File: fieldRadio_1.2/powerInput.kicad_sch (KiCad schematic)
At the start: 7 parts, among them Q21 IRF9540, U10 LM1086-5.0

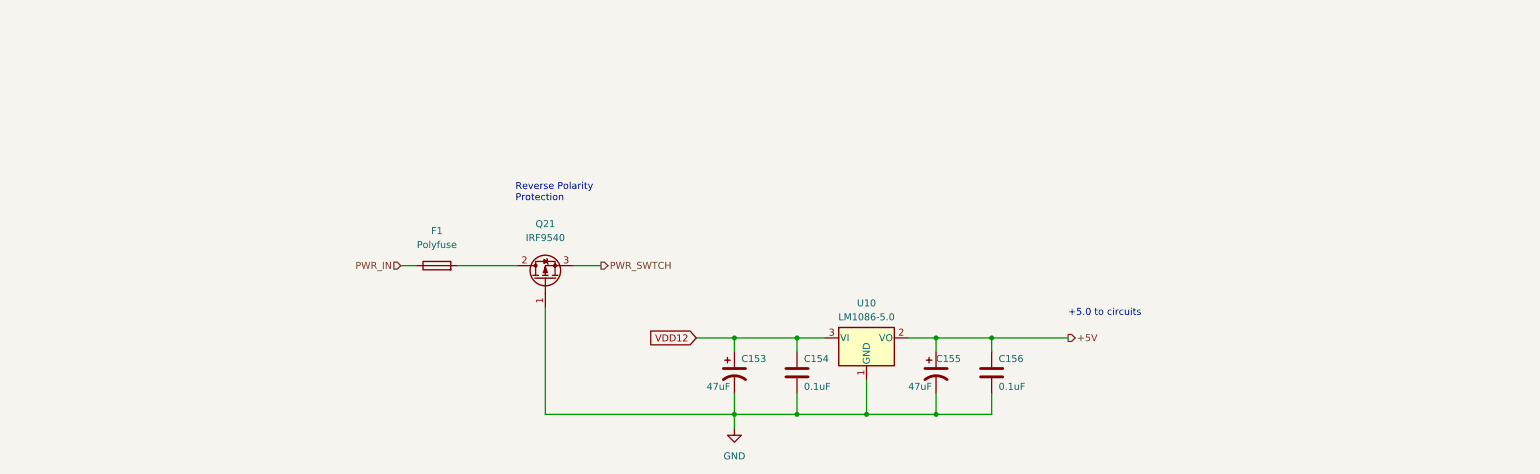
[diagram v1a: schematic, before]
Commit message: Working on fieldRadio_1.2 schematics
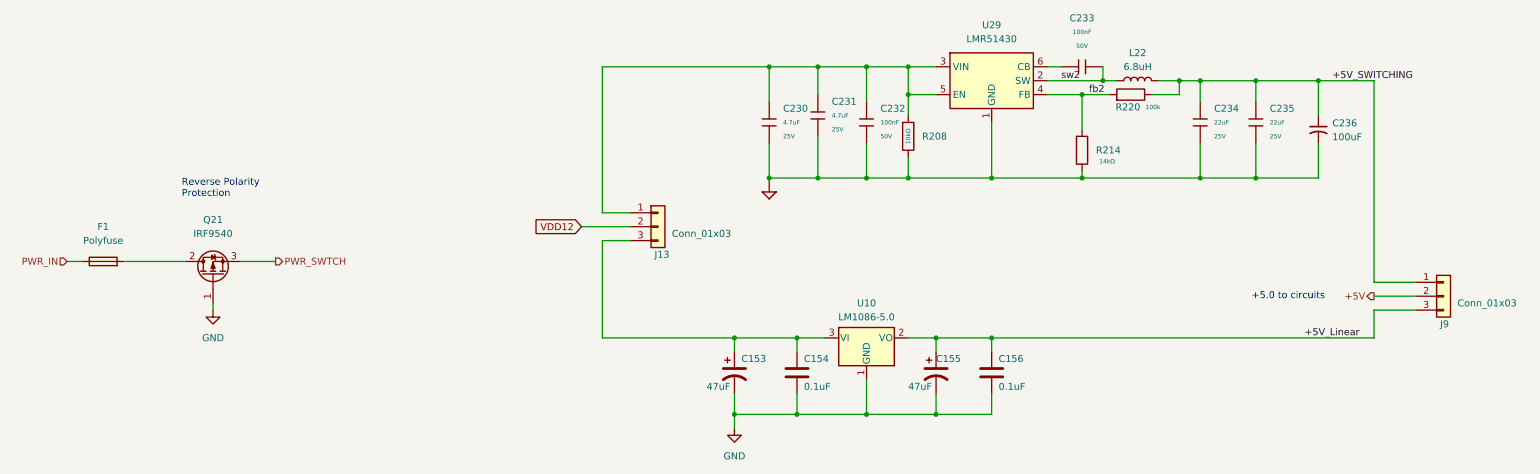
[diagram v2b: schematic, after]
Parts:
- added C230, C231: 4.7uF, PCM_JLCPCB:C_0805, symbol PCM_JLCPCB-Capacitors:0805,4.7uF
- added C232, C233: 100nF, PCM_JLCPCB:C_0603, symbol PCM_JLCPCB-Capacitors:0603,100nF
- added C234, C235: 22uF, PCM_JLCPCB:C_0805, symbol PCM_JLCPCB-Capacitors:0805,22uF
- added C236: 100uF, Capacitor_SMD:C_Elec_6.3x5.8, symbol Device:C_Small_US
- added J13, J9: Conn_01x03, Connector_Wire:SolderWire-0.75sqmm_1x03_P4.8mm_D1.25mm_OD2.3mm, symbol Connector_Generic:Conn_01x03
- added L22: 6.8uH, Inductor_SMD:L_TechFuse_SL0624, symbol Device:L
- added R208: 10kΩ, PCM_JLCPCB:R_0603, symbol PCM_JLCPCB-Resistors:0603,10kΩ
- added R214: 14kΩ, PCM_JLCPCB:R_0603, symbol PCM_JLCPCB-Resistors:0603,30kΩ
- added R220: 100k, PCM_JLCPCB:R_0603, symbol PCM_JLCPCB-Resistors:0603,10kΩ
- added U29: LMR51430, Package_TO_SOT_SMD:SOT-23-6, symbol Regulator_Switching:LMR51430
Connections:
- net +5V: now also J9.2 (Pin_2); no longer C155.1, C156.1, U10.2 (VO)
- net GND: now also C230.2, C231.2, C232.2, C234.2, C235.2, C236.2, R208.2, R214.2, U29.1 (GND)
- net VDD12: now also J13.2 (Pin_2); no longer C153.1, C154.1, U10.3 (VI)
- net at Q21.2 (D): no longer F1.2
- new net: C230.1, C231.1, C232.1, J13.1 (Pin_1), R208.1, U29.3 (VIN), U29.5 (EN)
- new net: C153.1, C154.1, J13.3 (Pin_3), U10.3 (VI)
- new net: C233.1, U29.6 (CB)
- new net +5V_Linear: C155.1, C156.1, J9.3 (Pin_3), U10.2 (VO)
- new net +5V_SWITCHING: C234.1, C235.1, C236.1, J9.1 (Pin_1), L22.2, R220.2
- new net fb2: R214.1, R220.1, U29.4 (FB)
- new net sw2: C233.2, L22.1, U29.2 (SW)
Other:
- moved on the sheet: F1, Q21
